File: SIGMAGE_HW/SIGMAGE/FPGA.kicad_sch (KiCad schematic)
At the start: 58 parts, among them J9 TSW10607GS, U41 MMBT2222A, U8 LFE5U25F6BG256I

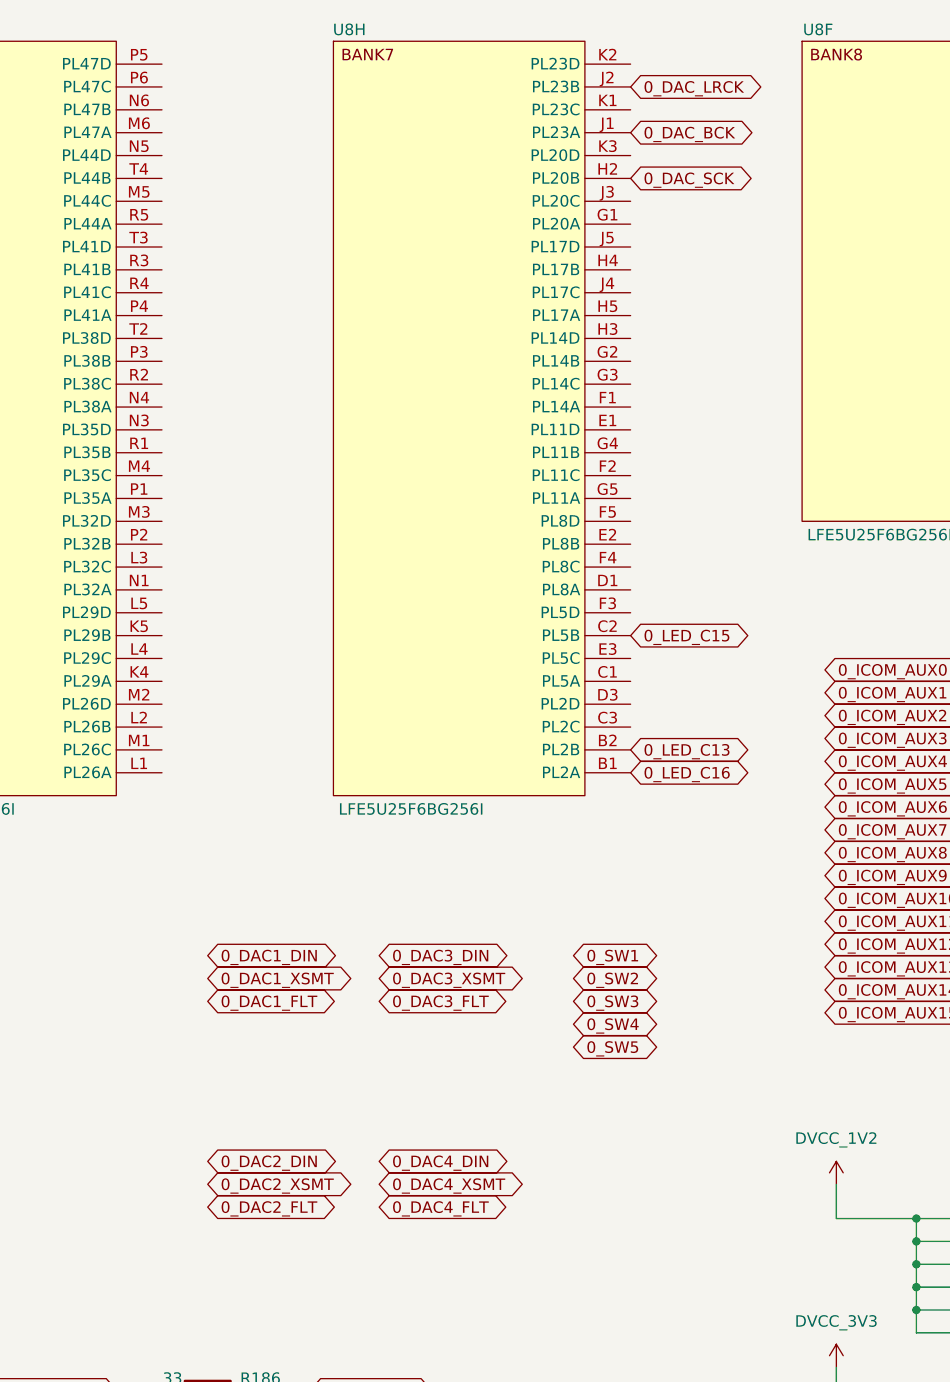
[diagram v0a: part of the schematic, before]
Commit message: foo bar
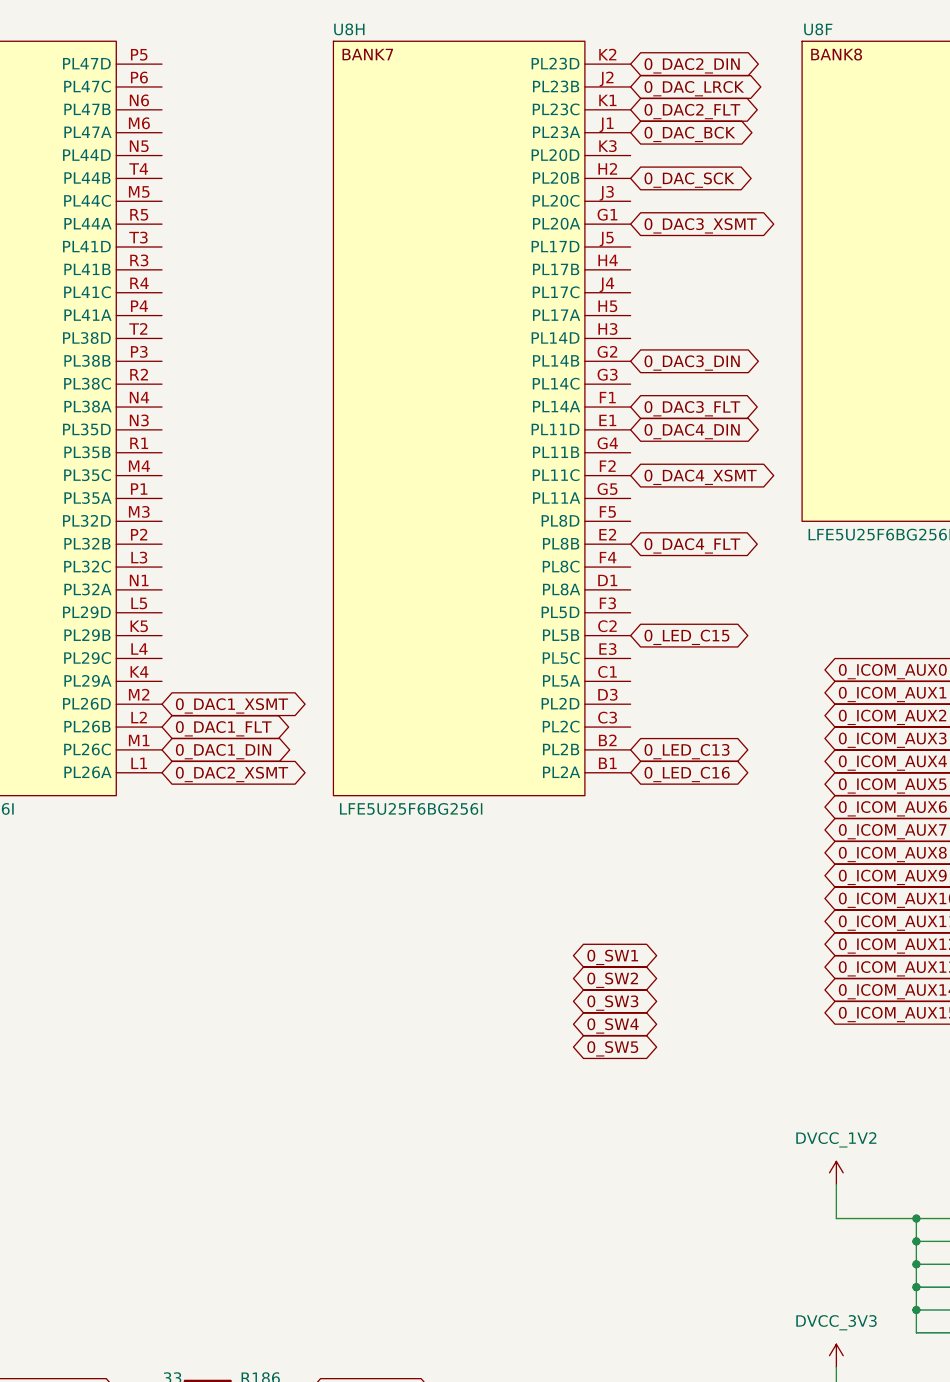
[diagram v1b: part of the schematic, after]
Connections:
- net 0_DAC1_DIN: now also U8.M1 (PL26C)
- net 0_DAC1_FLT: now also U8.L2 (PL26B)
- net 0_DAC1_XSMT: now also U8.M2 (PL26D)
- net 0_DAC2_DIN: now also U8.K2 (PL23D)
- net 0_DAC2_FLT: now also U8.K1 (PL23C)
- net 0_DAC2_XSMT: now also U8.L1 (PL26A)
- net 0_DAC3_DIN: now also U8.G2 (PL14B)
- net 0_DAC3_FLT: now also U8.F1 (PL14A)
- net 0_DAC3_XSMT: now also U8.G1 (PL20A)
- net 0_DAC4_DIN: now also U8.E1 (PL11D)
- net 0_DAC4_FLT: now also U8.E2 (PL8B)
- net 0_DAC4_XSMT: now also U8.F2 (PL11C)

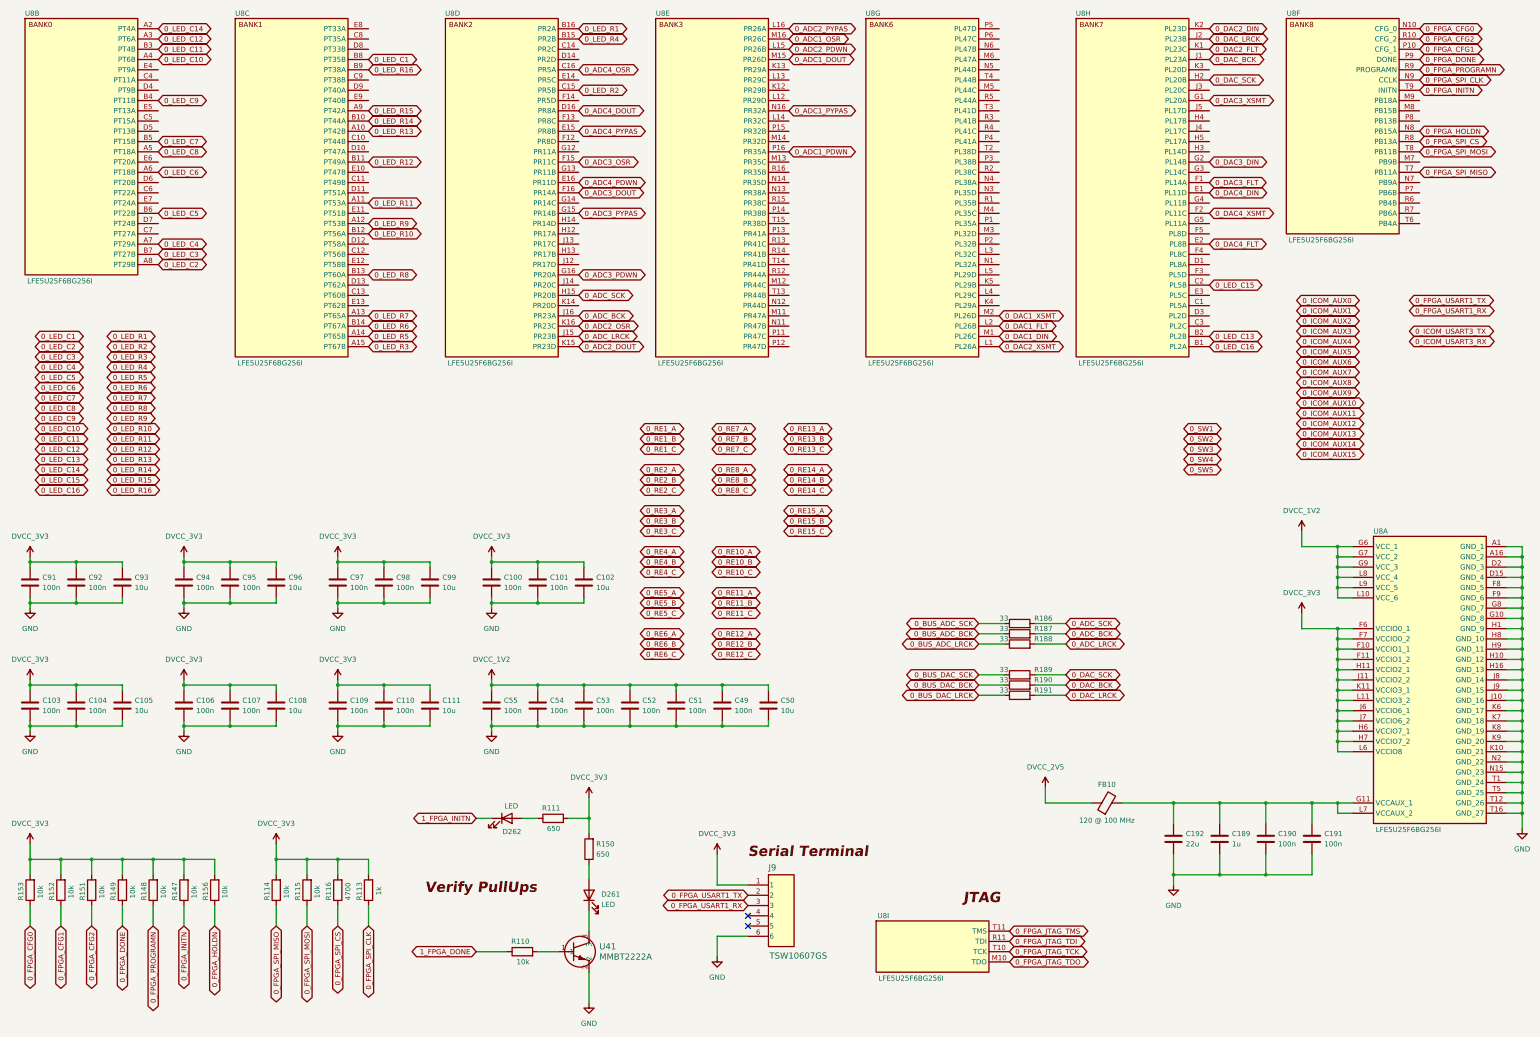
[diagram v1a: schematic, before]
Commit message: more routing
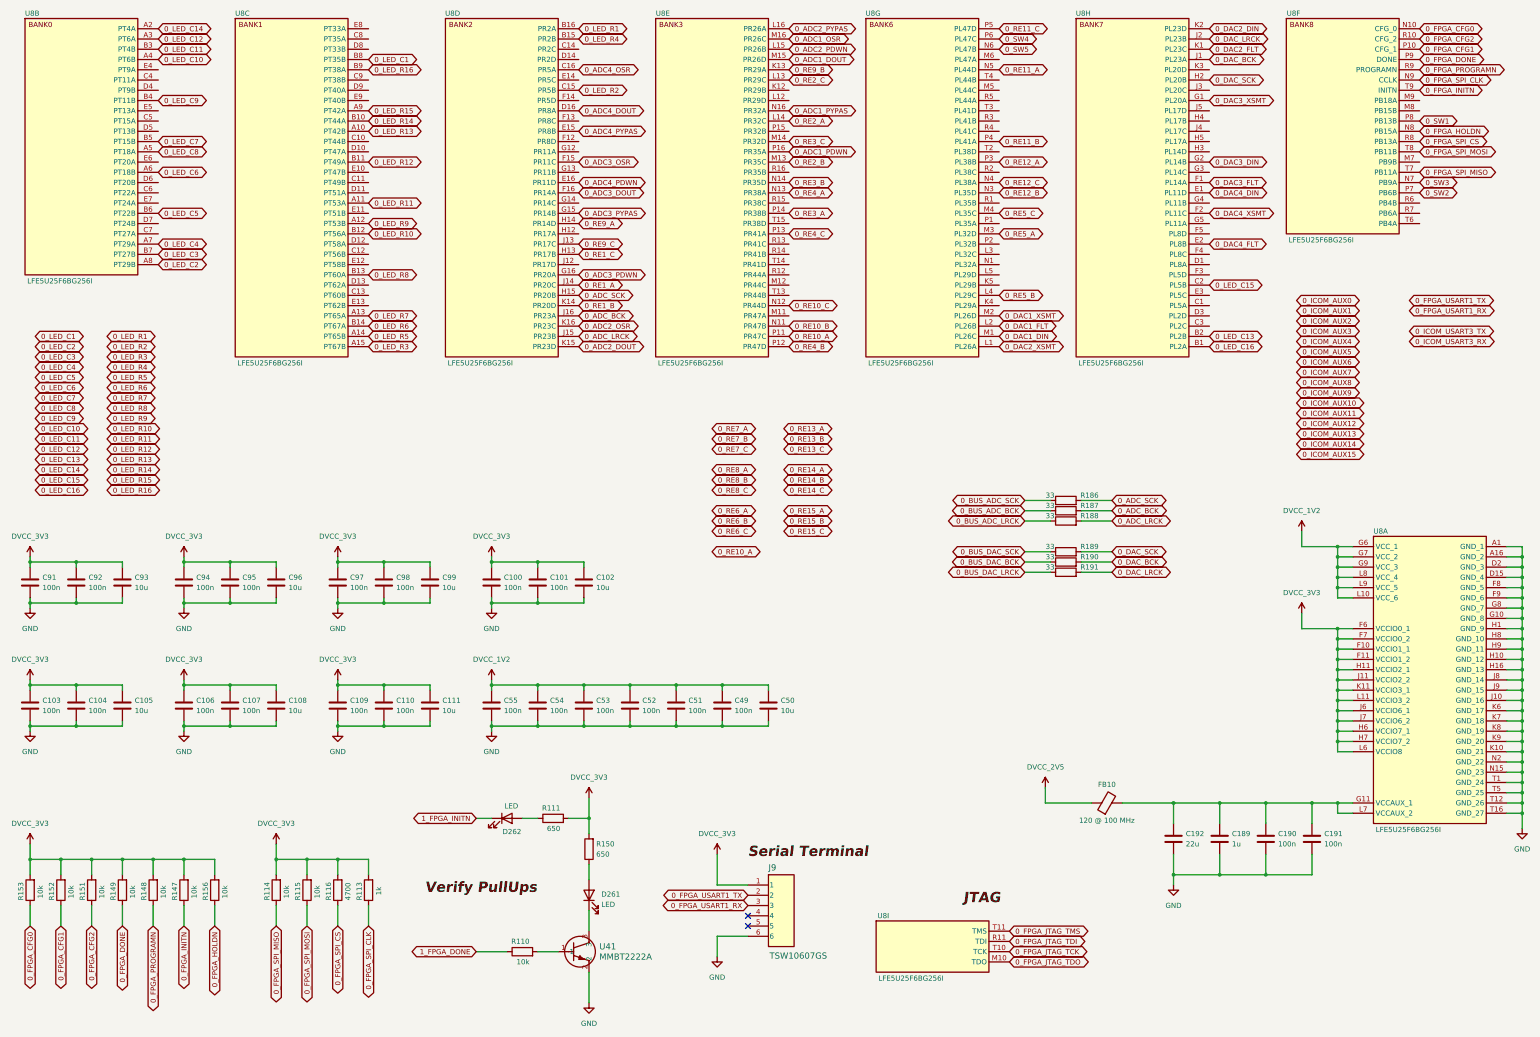
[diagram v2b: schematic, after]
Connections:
- net 0_RE10_A: now also U8.P11 (PR47C)
- net 0_RE10_B: now also U8.N11 (PR47B)
- net 0_RE10_C: now also U8.N12 (PR44D)
- net 0_RE11_A: now also U8.N5 (PL44D)
- net 0_RE11_B: now also U8.P4 (PL41A)
- net 0_RE11_C: now also U8.P5 (PL47D)
- net 0_RE12_A: now also U8.P3 (PL38B)
- net 0_RE12_B: now also U8.N3 (PL35D)
- net 0_RE12_C: now also U8.N4 (PL38A)
- net 0_RE1_A: now also U8.J14 (PR20C)
- net 0_RE1_B: now also U8.K14 (PR20D)
- net 0_RE1_C: now also U8.H13 (PR17B)
- net 0_RE2_A: now also U8.L14 (PR32C)
- net 0_RE2_B: now also U8.M13 (PR35C)
- net 0_RE2_C: now also U8.L13 (PR29C)
- net 0_RE3_A: now also U8.P14 (PR38B)
- net 0_RE3_B: now also U8.N14 (PR35D)
- net 0_RE3_C: now also U8.M14 (PR32D)
- net 0_RE4_A: now also U8.N13 (PR38A)
- net 0_RE4_B: now also U8.P12 (PR47D)
- net 0_RE4_C: now also U8.P13 (PR41A)
- net 0_RE5_A: now also U8.M3 (PL32D)
- net 0_RE5_B: now also U8.L4 (PL29C)
- net 0_RE5_C: now also U8.M4 (PL35C)
- net 0_SW1: now also U8.P8 (PB13B)
- net 0_SW2: now also U8.P7 (PB6B)
- net 0_SW3: now also U8.N7 (PB9A)
- net 0_SW4: now also U8.P6 (PL47C)
- net 0_SW5: now also U8.N6 (PL47B)
- net 0_RE9_B: now reaches U8.K13 (PR29A)
- net 0_RE9_A: now reaches U8.H14 (PR14D)
- net 0_RE9_C: now reaches U8.J13 (PR17C)
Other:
- moved on the sheet: R186, R187, R188, R189, R190, R191

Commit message: kek
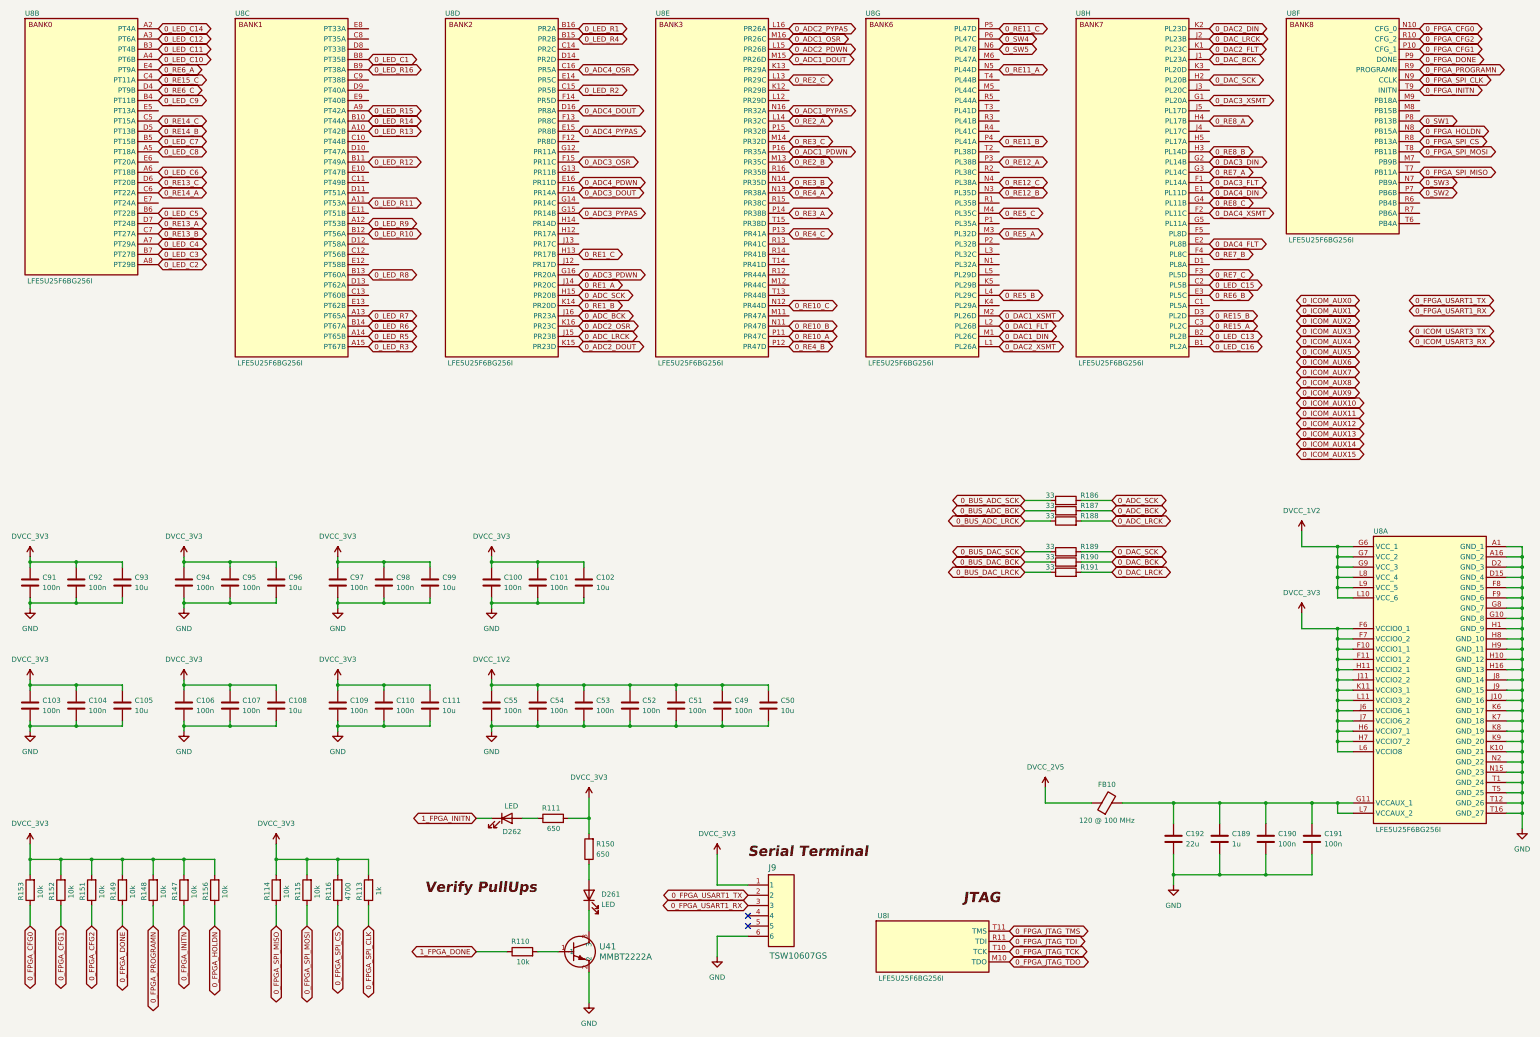
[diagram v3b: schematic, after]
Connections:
- net 0_RE13_A: now also U8.D7 (PT24B)
- net 0_RE13_B: now also U8.C7 (PT27A)
- net 0_RE13_C: now also U8.D6 (PT20B)
- net 0_RE14_A: now also U8.C6 (PT22A)
- net 0_RE14_B: now also U8.D5 (PT13B)
- net 0_RE14_C: now also U8.C5 (PT15A)
- net 0_RE15_A: now also U8.C3 (PL2C)
- net 0_RE15_B: now also U8.D3 (PL2D)
- net 0_RE15_C: now also U8.C4 (PT11A)
- net 0_RE6_A: now also U8.E4 (PT9A)
- net 0_RE6_B: now also U8.E3 (PL5C)
- net 0_RE6_C: now also U8.D4 (PT9B)
- net 0_RE7_A: now also U8.G3 (PL14C)
- net 0_RE7_B: now also U8.F4 (PL8C)
- net 0_RE7_C: now also U8.F3 (PL5D)
- net 0_RE8_A: now also U8.H4 (PL17B)
- net 0_RE8_B: now also U8.H3 (PL14D)
- net 0_RE8_C: now also U8.G4 (PL11B)
- net 0_RE9_A: no longer names the net of U8.H14 (PR14D)
- net 0_RE9_B: no longer names the net of U8.K13 (PR29A)
- net 0_RE9_C: no longer names the net of U8.J13 (PR17C)

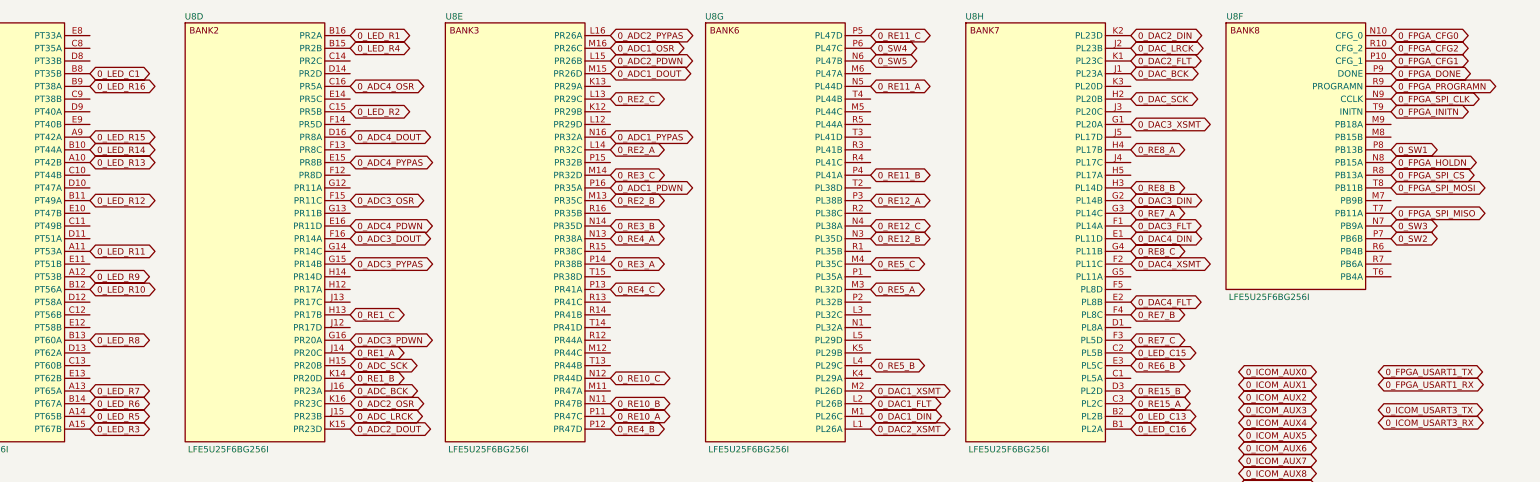
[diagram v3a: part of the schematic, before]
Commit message: shitty power traces part one
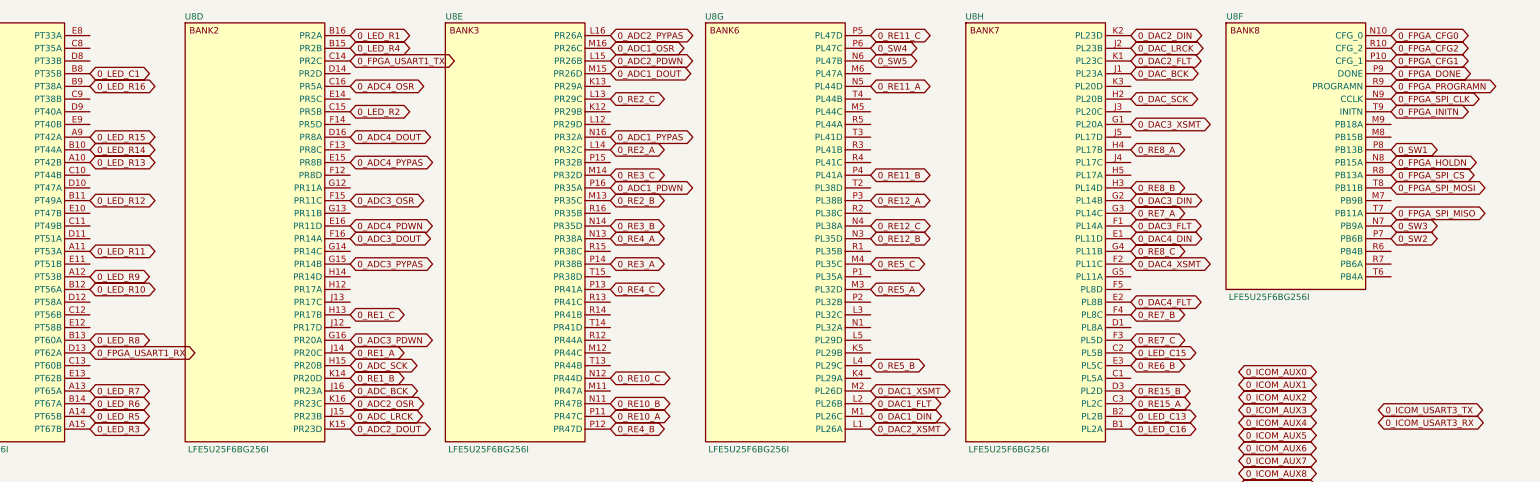
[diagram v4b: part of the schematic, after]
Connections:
- net 0_FPGA_USART1_RX: now also U8.D13 (PT62A)
- net 0_FPGA_USART1_TX: now also U8.C14 (PR2C)
